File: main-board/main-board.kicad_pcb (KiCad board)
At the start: 4 copper layers, 179 parts, among them IC10 SN74AXC4T774RSVR, IC13 TPS2121RUXR, IC15 SN74AXC4T774RSVR, IC16 SN74AXC4T774RSVR, IC2 SN74AXC4T774RSVR, IC3 SN74AXC4T774RSVR, IC4 SN74AXC4T774RSVR, J1 Conn_01x08, J12 Conn_01x01_Socket, J2 Conn_01x08, J37 Conn_01x03, J4 Conn_01x08, J47 Barrel Jack, J5 Conn_01x08, J66 Conn_01x01_Socket, J68 Conn_02x02_Odd_Even, J70 Conn_01x07, J71 Conn_02x01, J72 Conn_01x07, J73 Conn_01x03, J74 Conn_Coaxial, J8 Conn_01x16, P2 USB Micro, SW1 SW_SPDT, SW2 SW_SPDT, SW3 SW_SPDT, SW5 SW_Push, U1 FT4232HL, U11 TS5A23159DGS, U12 TS5A23159DGS, U13 TS5A23159DGS, U14 TS5A23159DGS, U17 74AHC244, U2 W25Q128JWSIQ, U24 TCA9554ADBQR, U27 SI5351A-B-GTR, U28 TS5A23159DGS, U3 TLV75801PDBV, U31 74AHC244, U9 74AHCT1G08, X2 OK322532.768KJBA4SL, Y1 Crystal_GND24, Y2 NX3225GA-25.000M-STD-CRG-2

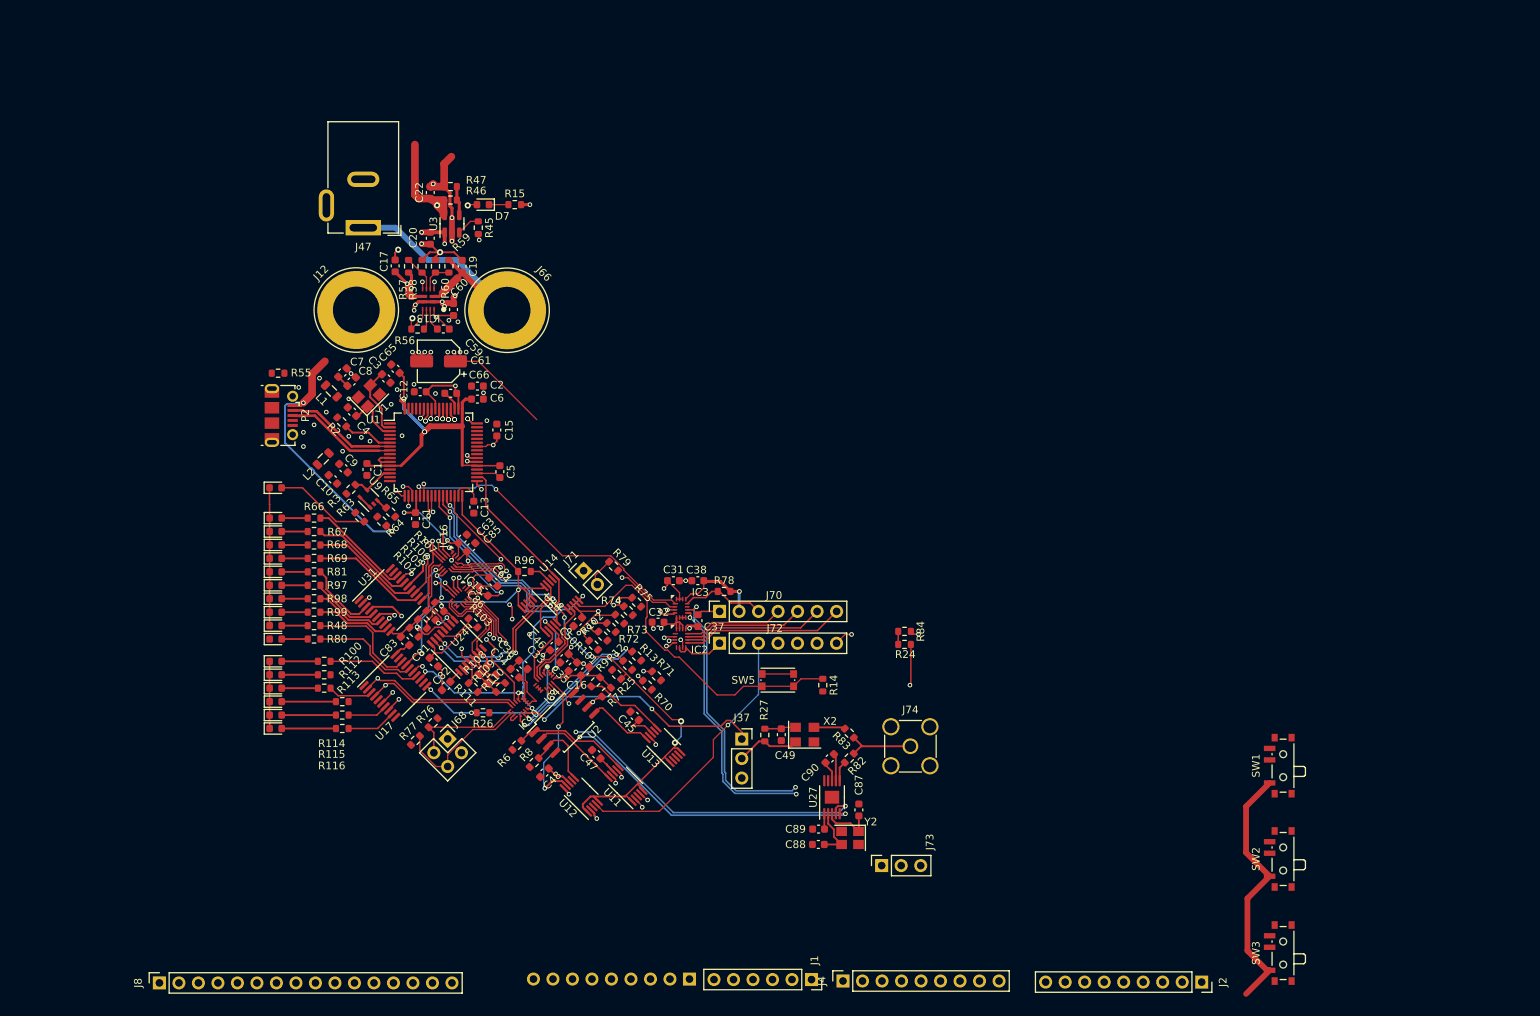
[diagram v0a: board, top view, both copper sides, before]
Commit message: First version of the chewing gum Vdc
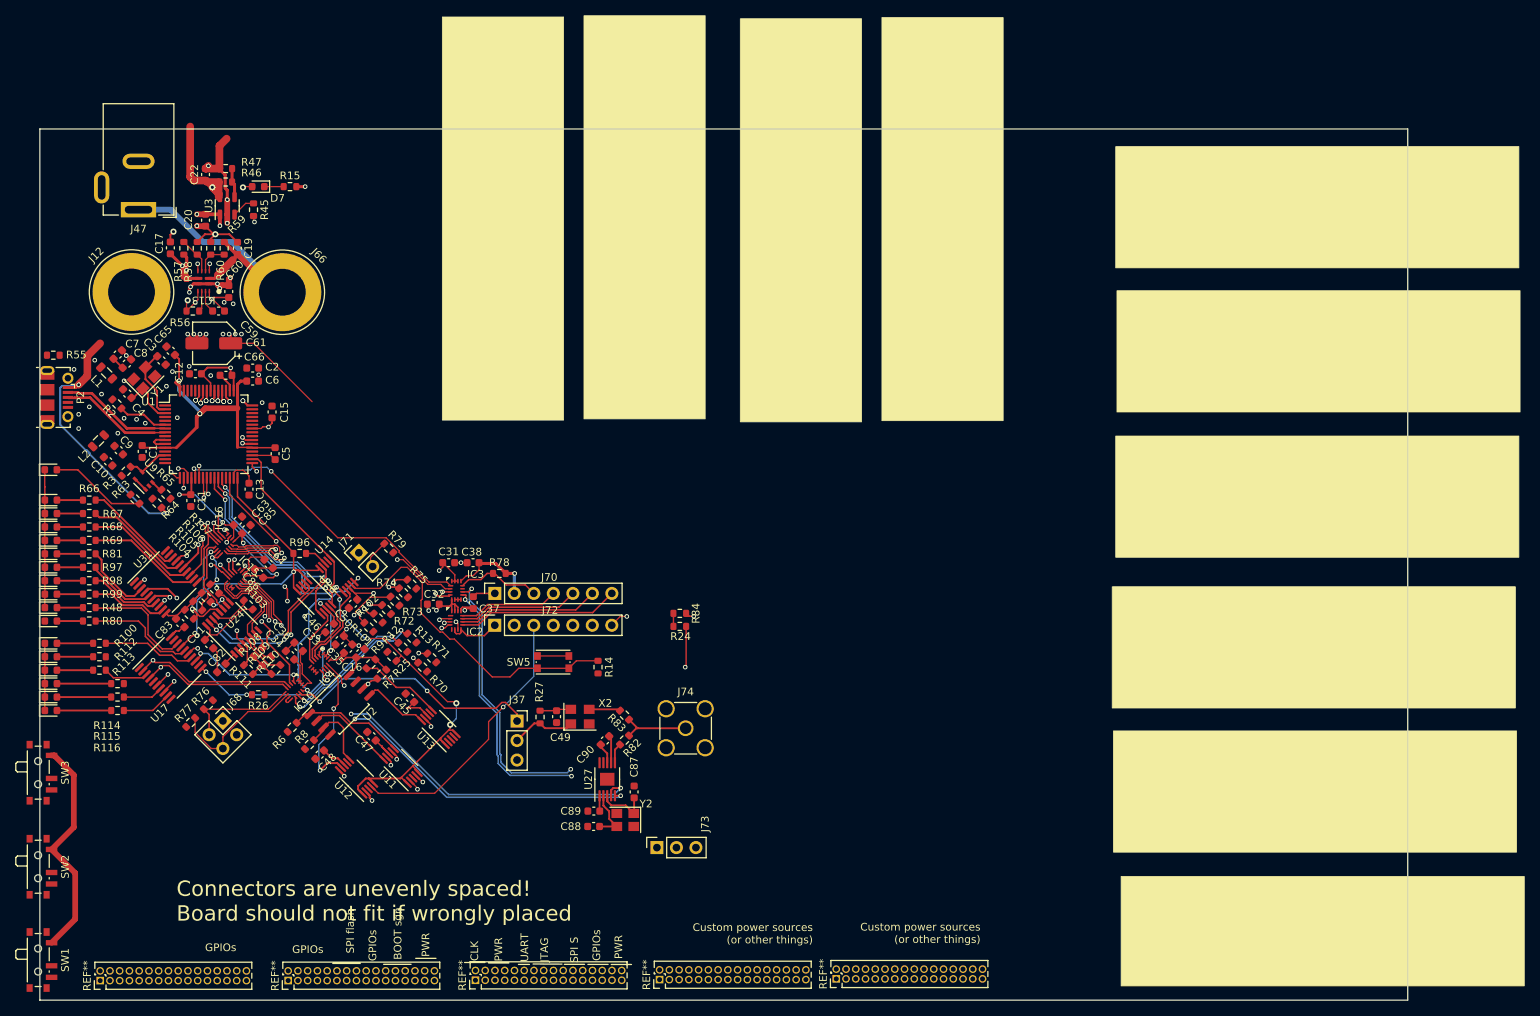
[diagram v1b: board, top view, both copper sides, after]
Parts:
- removed J1: Conn_01x08, Connector_PinSocket_2.54mm:PinSocket_1x06_P2.54mm_Vertical
- removed J2, J4, J5: Conn_01x08, Connector_PinSocket_2.54mm:PinSocket_1x09_P2.54mm_Vertical
- removed J8: Conn_01x16, Connector_PinSocket_2.54mm:PinSocket_1x16_P2.54mm_Vertical
- added REF**: PinHeader_2x16_P1.27mm_Vertical, Connector_PinHeader_1.27mm:PinHeader_2x16_P1.27mm_Vertical, F.Cu at (78.1, 148.8)
- added REF**: PinHeader_2x16_P1.27mm_Vertical, Connector_PinHeader_1.27mm:PinHeader_2x16_P1.27mm_Vertical, F.Cu at (173.9, 148.6)
- added REF**: PinHeader_2x16_P1.27mm_Vertical, Connector_PinHeader_1.27mm:PinHeader_2x16_P1.27mm_Vertical, F.Cu at (102.6, 148.8)
- added REF**: PinHeader_2x16_P1.27mm_Vertical, Connector_PinHeader_1.27mm:PinHeader_2x16_P1.27mm_Vertical, F.Cu at (150.9, 148.7)
- added REF**: PinHeader_2x16_P1.27mm_Vertical, Connector_PinHeader_1.27mm:PinHeader_2x16_P1.27mm_Vertical, F.Cu at (127.0, 148.7)
- moved SW1 163.5 mm to (70.3, 146.1), turned to -90 degrees
- moved SW3 163.2 mm to (70.3, 121.7), turned to -90 degrees
- moved SW2 161.5 mm to (70.3, 134.0), turned to -90 degrees
- moved C16 29.4 mm to (112.0, 106.2)
- moved IC4 29.4 mm to (106.7, 107.5)
- moved Y2 29.4 mm to (146.5, 127.9)
- moved C1 29.4 mm to (83.5, 79.9)
- moved C11 29.4 mm to (89.9, 86.3)
- moved C12 29.4 mm to (90.5, 69.8)
- moved C15 29.4 mm to (100.5, 74.7)
- moved C17 29.4 mm to (87.2, 53.4)
- moved C2 29.4 mm to (97.9, 69.0)
- moved C20 29.4 mm to (91.8, 49.8)
- moved C22 29.4 mm to (91.8, 43.8)
- moved C31 29.4 mm to (123.5, 94.4)
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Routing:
- net /V_IO: track 97.6 -> 93.3 mm
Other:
- board outline added: 178.1 x 113.5 mm
- board text added: "BOOT sgn"
- board text added: "CLK"
- board text added: "Connectors are unevenly spaced! Board should not fit if wrongly placed"
- board text added: "Custom power sources (or other things)"
- board text added: "GPIOs"
- board text added: "JTAG"
- board text added: "PWR"
- board text added: "SPI S"
- board text added: "UART"
